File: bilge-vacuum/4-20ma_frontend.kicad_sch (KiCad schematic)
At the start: 6 parts, among them J2 Screw_Terminal_01x02, U10 MAX14626, U11 LMV321

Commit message: Vac progress
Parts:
- J2: footprint (none) -> Custom Parts:2604-1102
- U11: footprint (none) -> Custom Parts:SOT23-5
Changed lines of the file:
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@@
       (effects (font (size 1.27 1.27)) (justify left))
     )
-    (property "Footprint" "" (at 55.245 43.18 0)
+    (property "Footprint" "Custom Parts:2604-1102" (at 55.245 43.18 0)
       (effects (font (size 1.27 1.27)) hide)
     )
@@
       (effects (font (size 1.27 1.27)))
     )
-    (property "Footprint" "" (at 86.995 71.12 0)
+    (property "Footprint" "Custom Parts:SOT23-5" (at 86.995 71.12 0)
       (effects (font (size 1.27 1.27)) (justify left) hide)
     )

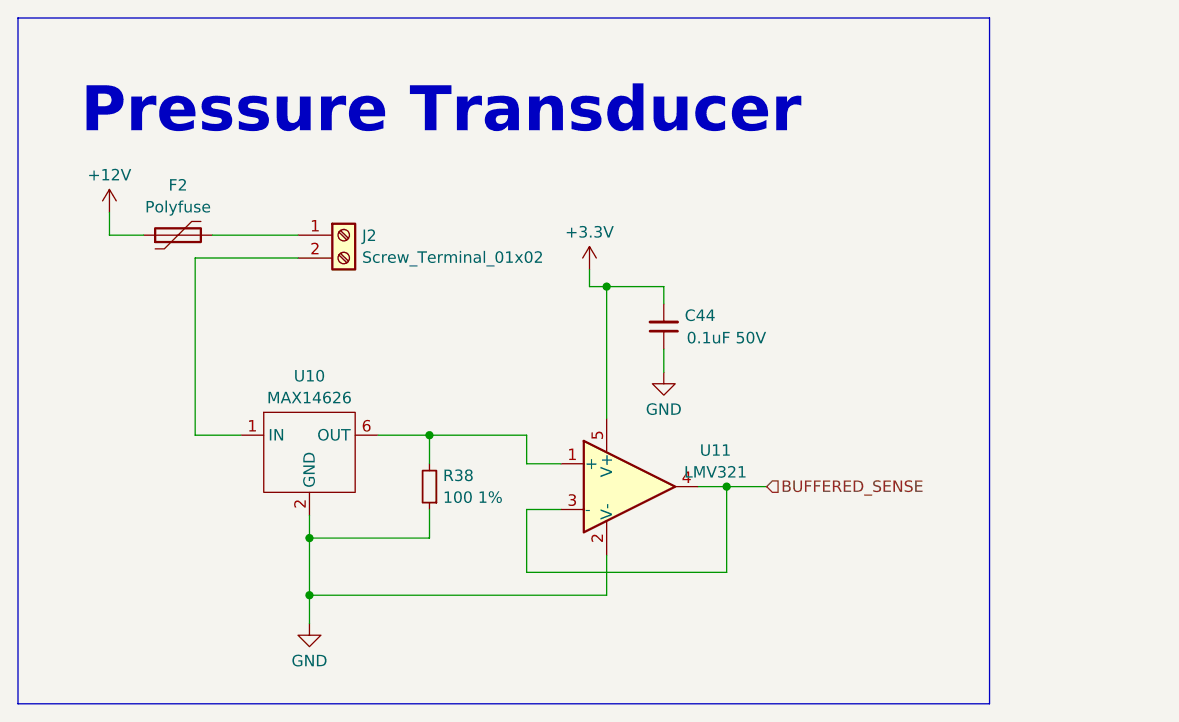
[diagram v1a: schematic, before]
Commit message: bilge vac 1v0
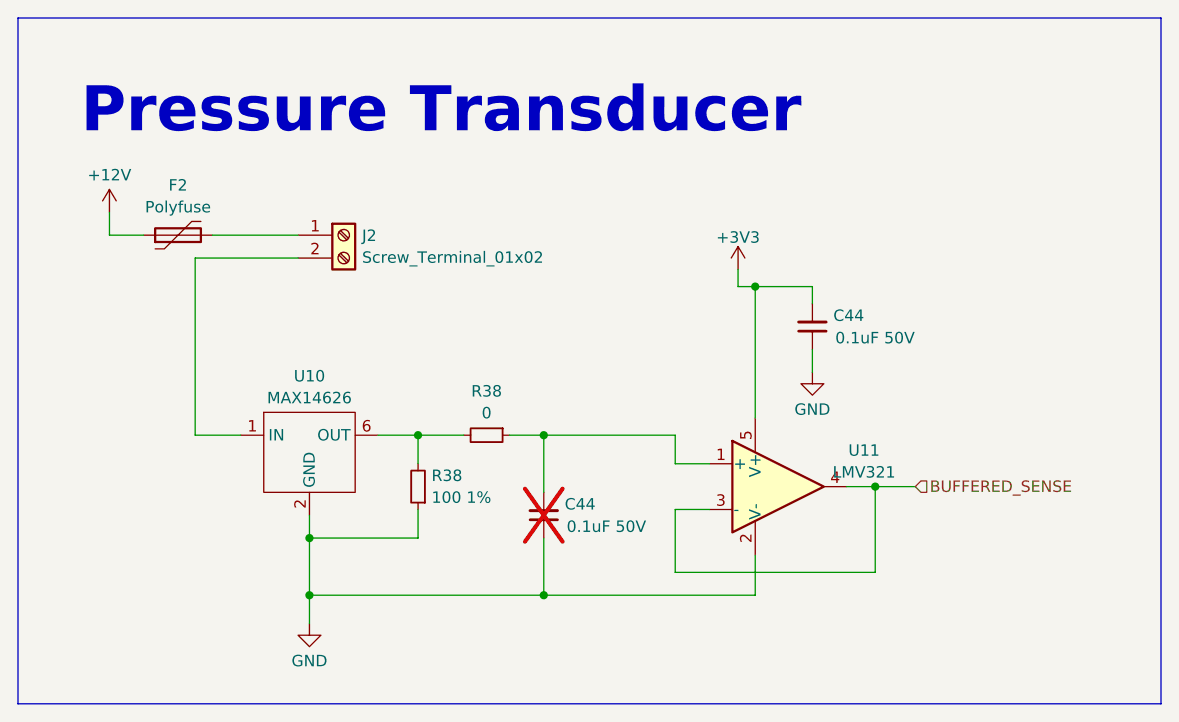
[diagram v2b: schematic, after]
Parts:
- added C44: 0.1uF 50V, Capacitor_SMD:C_0805_2012Metric, symbol Device:C_Small
- added R38: 0, Resistor_SMD:R_0805_2012Metric, symbol Device:R_Small
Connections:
- net GND: now also C44.1
- net at R38.2, U10.6 (OUT): now also R38.2; no longer U11.1 (+)
- net +3.3V renamed +3V3
- new net: C44.2, R38.1, U11.1 (+)
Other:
- moved on the sheet: C44, R38, U11

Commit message: Fixes
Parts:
- F2: footprint Resistor_SMD:R_2010_5025Metric -> Custom Parts:SMD_2016
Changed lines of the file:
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@@
       (effects (font (size 1.27 1.27)))
     )
-    (property "Footprint" "Resistor_SMD:R_2010_5025Metric" (at 41.91 41.91 0)
+    (property "Footprint" "Custom Parts:SMD_2016" (at 41.91 41.91 0)
       (effects (font (size 1.27 1.27)) (justify left) hide)
     )
